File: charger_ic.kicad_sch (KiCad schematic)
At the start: 9 parts, among them J1 USB_C_Receptacle, U5 TPS25730D, U6 BQ25798, U7 TVS2200DRV

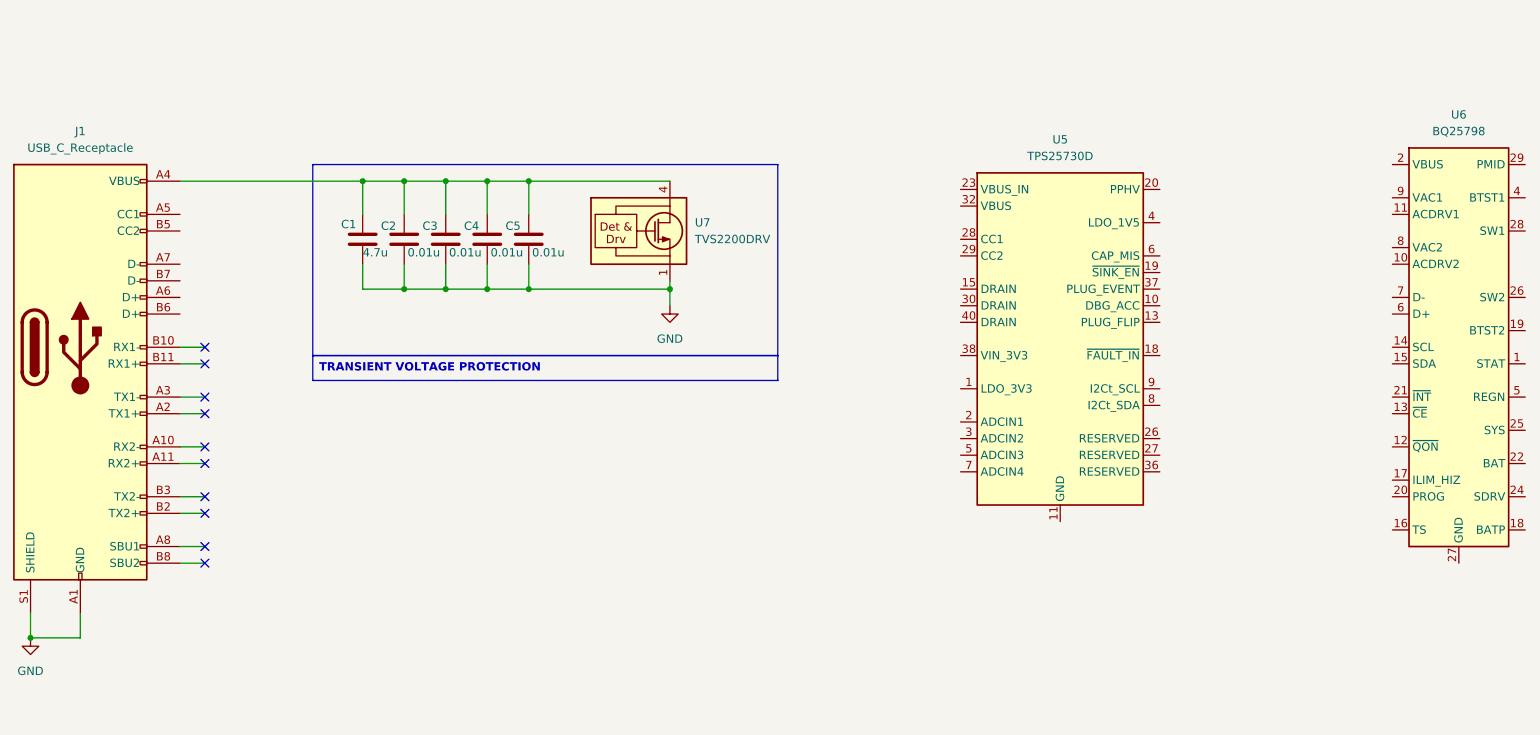
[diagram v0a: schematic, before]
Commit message: usb pd charging
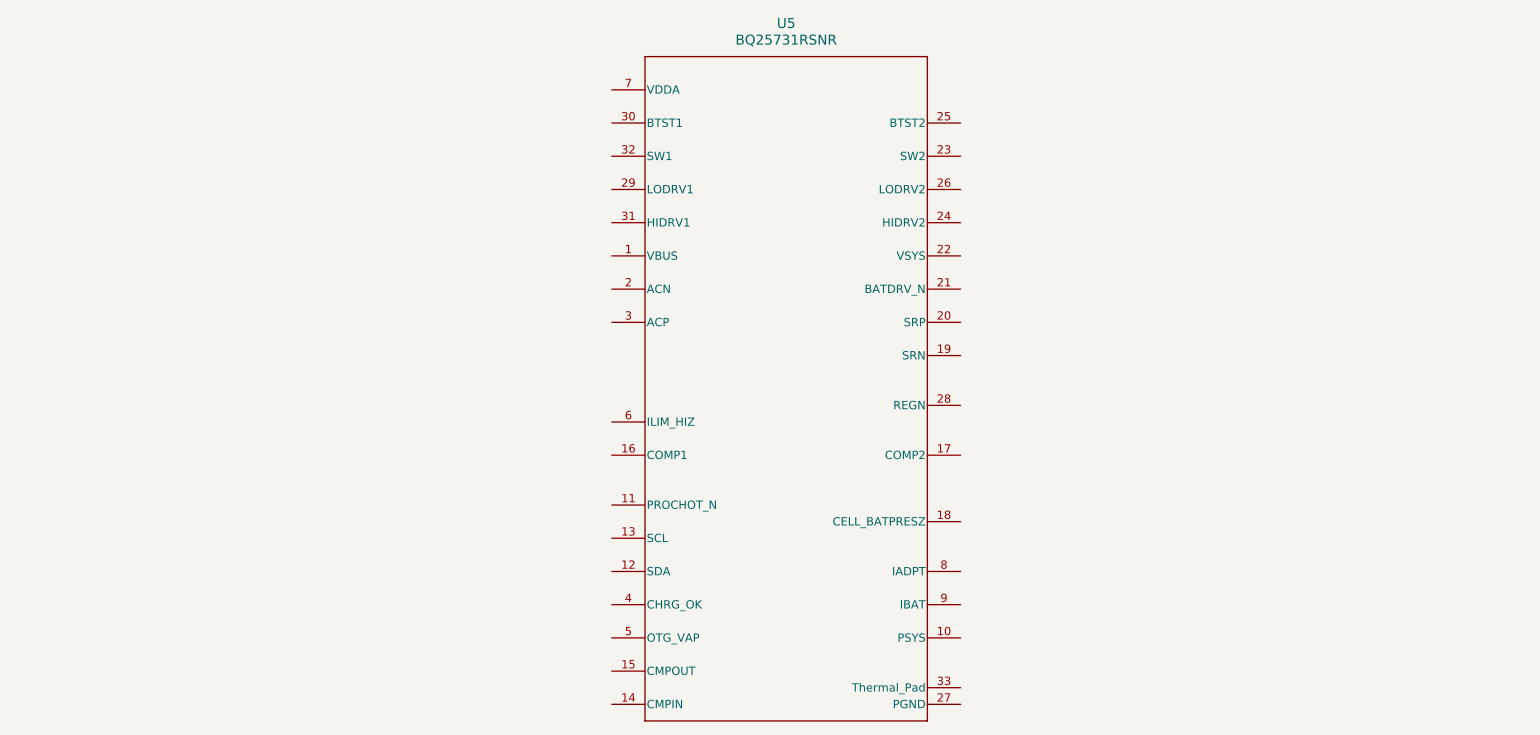
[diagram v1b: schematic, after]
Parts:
- removed C1: 4.7u, symbol Device:C
- removed C2, C3, C4, C5: 0.01u, symbol Device:C
- removed J1: USB_C_Receptacle, symbol Connector:USB_C_Receptacle
- removed U5: TPS25730D, Package_DFN_QFN:Texas_REF0038A_WQFN-38-2EP_6x4mm_P0.4, symbol Interface_USB:TPS25730D
- removed U6: BQ25798, Package_DFN_QFN:Texas_RQM0029A_VQFN-29_4x4mm_P0.4mm, symbol Battery_Management:BQ25798
- removed U7: TVS2200DRV, Package_SON:WSON-6-1EP_2x2mm_P0.65mm_EP1x1.6mm, symbol Power_Protection:TVS2200DRV
- added U5: BQ25731RSNR, RSN0032B-IPC_A, symbol BQ25731RSNR:BQ25731RSNR
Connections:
- no-connect marks 10 -> 0
